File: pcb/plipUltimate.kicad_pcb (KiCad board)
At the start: 2 copper layers, 50 x 50 mm, 55 parts, among them CON1 IEEEE-1284A, CON2 AVR-ISP-6, CON3 RJ45_C, CON4 SD_SPI, CON5 USB_microB, U1 ENC28J60, U2 ATMEGA328P, U3 LM2596_5.0, U4 74LS07, U5 IRF7309, U6 AMS1117_3V3, U7 IRF7309, X1 25MHz

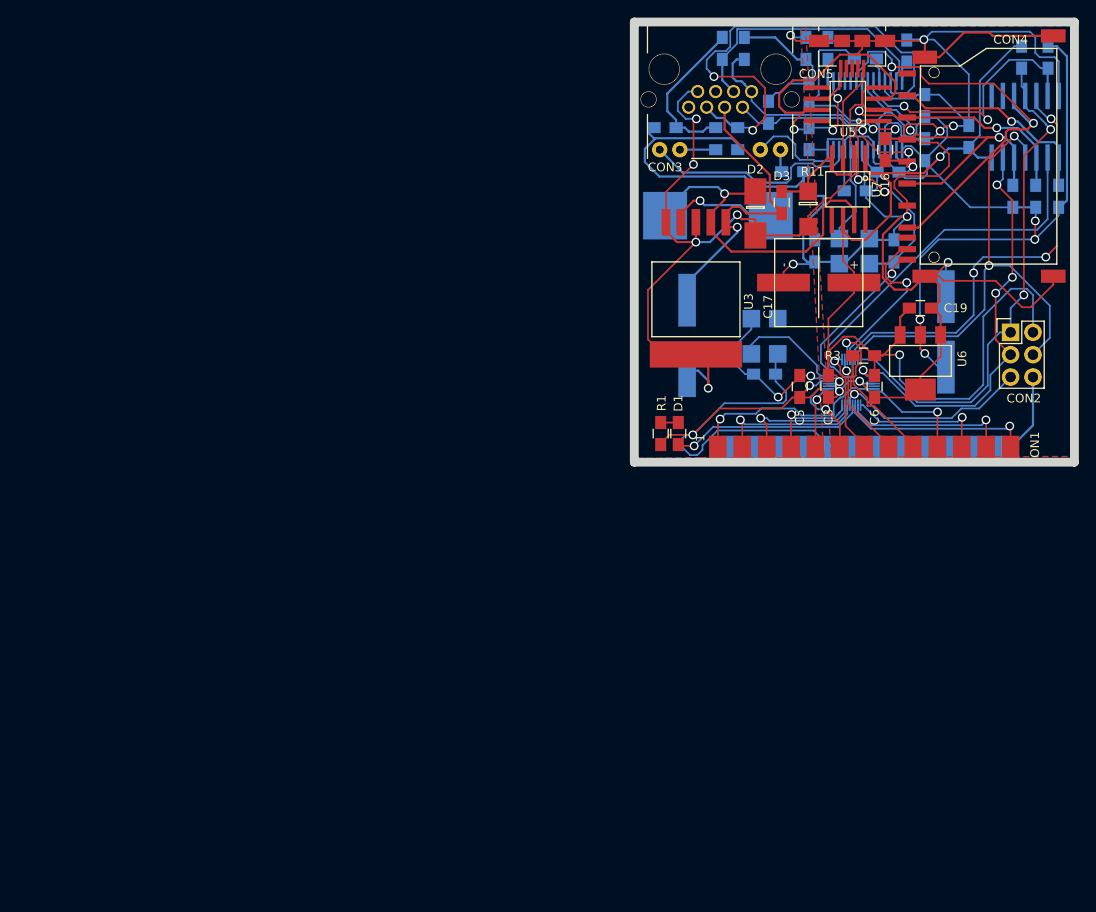
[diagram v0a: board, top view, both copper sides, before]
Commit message: Revised schematic, reroute in progress
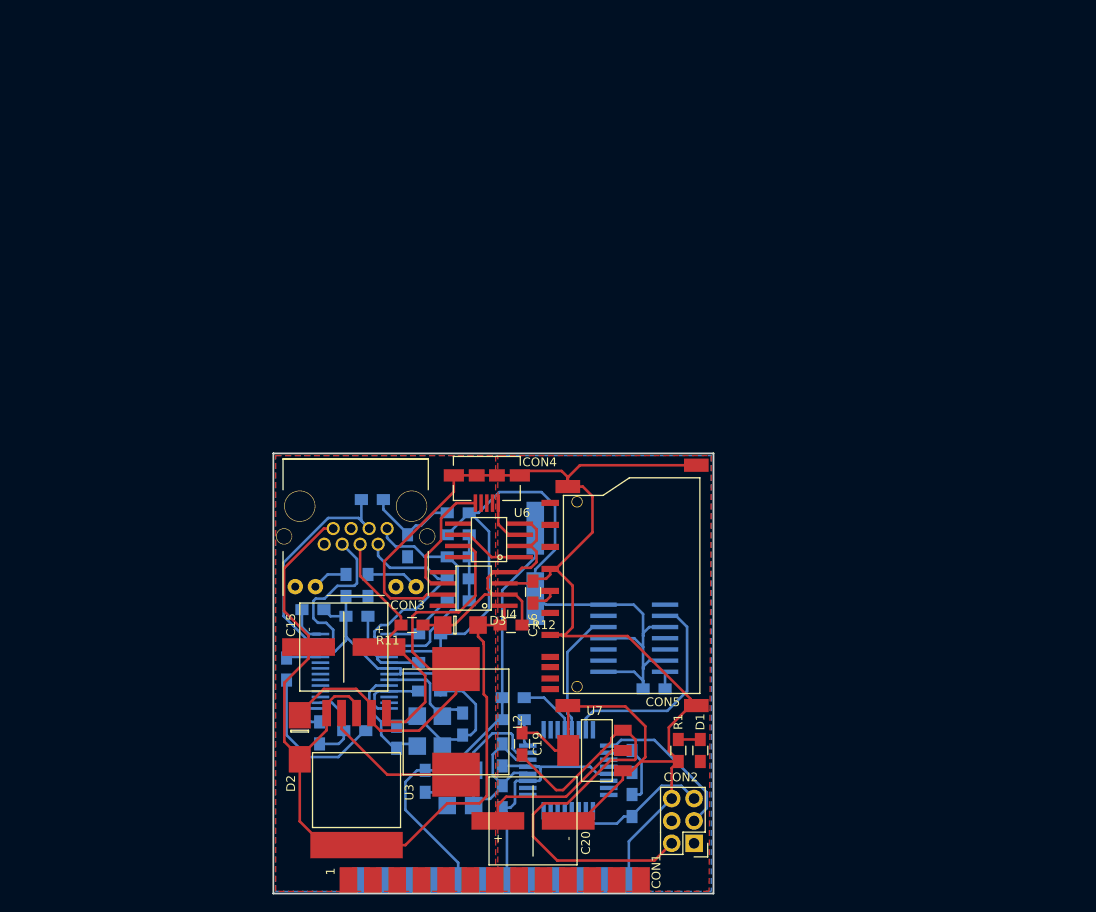
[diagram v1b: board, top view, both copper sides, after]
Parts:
- removed R15, R16: 1k, plipUltimate:0805
- C15, C20, L2: moved to F.Cu
- C17: value 220uF 35V loESR -> 10nF; footprint plipUltimate:electrolyte_SMD -> plipUltimate:0805; moved to B.Cu
- C18: value 10nF -> 220uF 35V loESR; footprint plipUltimate:0805 -> plipUltimate:electrolyte_SMD
- C3, C5, C6, R3: moved to B.Cu
- CON4: value SD_SPI -> USB_microB; footprint plipUltimate:SD-SHORT -> plipUltimate:USB-MicroB
- CON5: value USB_microB -> SD_SPI; footprint plipUltimate:USB-MicroB -> plipUltimate:SD-SHORT
- R1: value 330R -> 820R
- R12: value 1k -> 10k; moved to F.Cu
- R13, R14: value 1k -> 4k7
- U2: footprint plipUltimate:TQFP_32 -> plipUltimate:TQFP-32
- U4: value 74LS07 -> IRF7309; footprint plipUltimate:SO-14 -> plipUltimate:SO-8; moved to F.Cu
- U5: value IRF7309 -> 74LVC125; footprint plipUltimate:SO-8 -> plipUltimate:SO-14; moved to B.Cu
- U6: value AMS1117_3V3 -> IRF7309; footprint plipUltimate:SOT-223 -> plipUltimate:SO-8
- U7: value IRF7309 -> AMS1117_3V3; footprint plipUltimate:SO-8 -> plipUltimate:SOT-223
- moved C8 96.9 mm to (84.2, 120.8), turned to 90 degrees
- moved R13 96.7 mm to (106.2, 119.2), turned to 0 degrees
- moved R4 95.5 mm to (80.5, 113.5), turned to 90 degrees
- moved R2 92.6 mm to (83.5, 106.8), turned to 0 degrees
- moved C2 86.7 mm to (88.5, 107.5), turned to 0 degrees
- moved R12 86.7 mm to (106.0, 108.5), turned to 0 degrees
- moved U1 85.7 mm to (88.2, 113.8), turned to 90 degrees
- moved C1 84.8 mm to (88.2, 120.5), turned to 0 degrees
- moved R14 84.1 mm to (106.2, 116.8), turned to 0 degrees
- moved U4 80.1 mm to (104.2, 106.3), turned to 90 degrees
- moved D2 78.9 mm to (82.0, 121.2)
- moved C4 78.7 mm to (96.8, 109.5), turned to 180 degrees
- moved CON5 78.2 mm to (111.5, 115.8), turned to 90 degrees
- moved C7 76.3 mm to (96.8, 112.8), turned to 180 degrees
- moved C9 74.6 mm to (96.8, 116.0)
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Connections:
- C17 pad 1: +5V -> +3V3
- C18 pad 1: GND -> +5V
- C18 pad 2: +5V -> GND
- CON4 pad 1: 3.3V_SD_CS -> Net-(CON4-Pad1)
- CON4 pad 2: 3.3V_AVR_MOSI -> Net-(CON4-Pad2)
- CON4 pad 3: GND -> Net-(CON4-Pad3)
- CON4 pad 4: +3V3 -> Net-(CON4-Pad4)
- CON4 pad 5: 3.3V_AVR_SCK -> Net-(CON4-Pad5)
- CON5 pad 1: Net-(CON5-Pad1) -> 3.3V_SD_CS
- CON5 pad 2: Net-(CON5-Pad2) -> 3.3V_AVR_MOSI
- CON5 pad 3: Net-(CON5-Pad3) -> GND
- CON5 pad 4: Net-(CON5-Pad4) -> +3V3
- CON5 pad 5: Net-(CON5-Pad5) -> 3.3V_AVR_SCK
- R12 pad 1: +5V -> POE_0V
- R12 pad 2: AVR_MISO -> Net-(D3-Pad1)
- R13 pad 1: +3V3 -> +5V
- R13 pad 2: 3.3V_ETH_CS -> SD_DETECT
- R14 pad 1: +3V3 -> +5V
- R14 pad 2: 3.3V_SD_CS -> SD_LOCK
- U1 pad 6: 3.3V_AVR_MISO -> AVR_MISO
- U1 pad 7: 3.3V_AVR_MOSI -> AVR_MOSI
- U1 pad 8: 3.3V_AVR_SCK -> AVR_SCK
- U1 pad 9: 3.3V_ETH_CS -> ETH_CS
- U4 pad 1: Net-(U4-Pad1) -> POE_0V
- U4 pad 2: Net-(U4-Pad2) -> Net-(D3-Pad1)
- U4 pad 3: 3.3V_AVR_MISO -> GND
- U4 pad 4: AVR_MISO -> Net-(D3-Pad1)
- U4 pad 5: ETH_CS -> (no net)
- U4 pad 6: 3.3V_ETH_CS -> Net-(CON4-Pad5)
- U4 pad 8: 3.3V_SD_CS -> (no net)
- U5 pad 1: POE_0V -> GND
- U5 pad 2: Net-(D3-Pad1) -> Net-(U5-Pad2)
- U5 pad 3: GND -> Net-(U5-Pad3)
- U5 pad 4: Net-(D3-Pad1) -> GND
- U5 pad 5: (no net) -> SD_CS
- U5 pad 6: Net-(CON5-Pad5) -> 3.3V_SD_CS
- U5 pad 8: (no net) -> 3.3V_AVR_MOSI
- U6 pad 1: GND -> +5V
- U6 pad 2: +3V3 -> Net-(D3-Pad1)
- U6 pad 3: +5V -> Net-(CON4-Pad1)
- U7 pad 1: +5V -> GND
- U7 pad 2: Net-(D3-Pad1) -> +3V3
- U7 pad 3: Net-(CON5-Pad1) -> +5V
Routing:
- net +3V3: track 150.2 -> 68.0 mm, vias 5 -> 0
- net AVR_MISO: track 58.9 -> 0.00 mm, vias 2 -> 0
- net 3.3V_AVR_MISO: track 51.6 -> 0.00 mm, vias 2 -> 0
- net ETH_CS: track 51.5 -> 0.00 mm, vias 3 -> 0
- net 3.3V_AVR_SCK: track 37.9 -> 0.00 mm, vias 2 -> 0
- net Net-(CON3-Pad6): track 56.3 -> 18.8 mm, vias 2 -> 0
- net AVR_MOSI: track 56.5 -> 24.4 mm, vias 2 -> 0
- net 3.3V_ETH_CS: track 31.7 -> 0.00 mm, vias 2 -> 0
- net SD_CS: track 45.2 -> 14.4 mm
- net 3.3V_AVR_MOSI: track 30.6 -> 0.00 mm, vias 2 -> 0
- net AVR_SCK: track 45.4 -> 18.7 mm, vias 3 -> 0
- net /~STROBE: track 26.6 -> 0.00 mm, vias 1 -> 0
- net GND: track 430.3 -> 404.5 mm, vias 14 -> 0
- net Net-(CON3-Pad12): track 25.2 -> 0.00 mm
- net 3.3V_SD_CS: track 24.0 -> 0.00 mm, vias 1 -> 0
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- added copper zone on B.Cu, net GND
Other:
- net class Default: clearance 0.1 -> 0.3; trace_width 0.2 -> 0.3; via_dia 1 -> 1.5; via_drill 0.7 -> 0.3
- rule pad_to_mask_clearance: 0.2 -> 0
- rule trace_clearance: 0.1 -> 0.3
- rule via_min_size: 1 -> 0.4
- board text added: "BS: Children of the grave Rev. 2"
- board text added: "github.com/tehKaiN/plipUltimate"

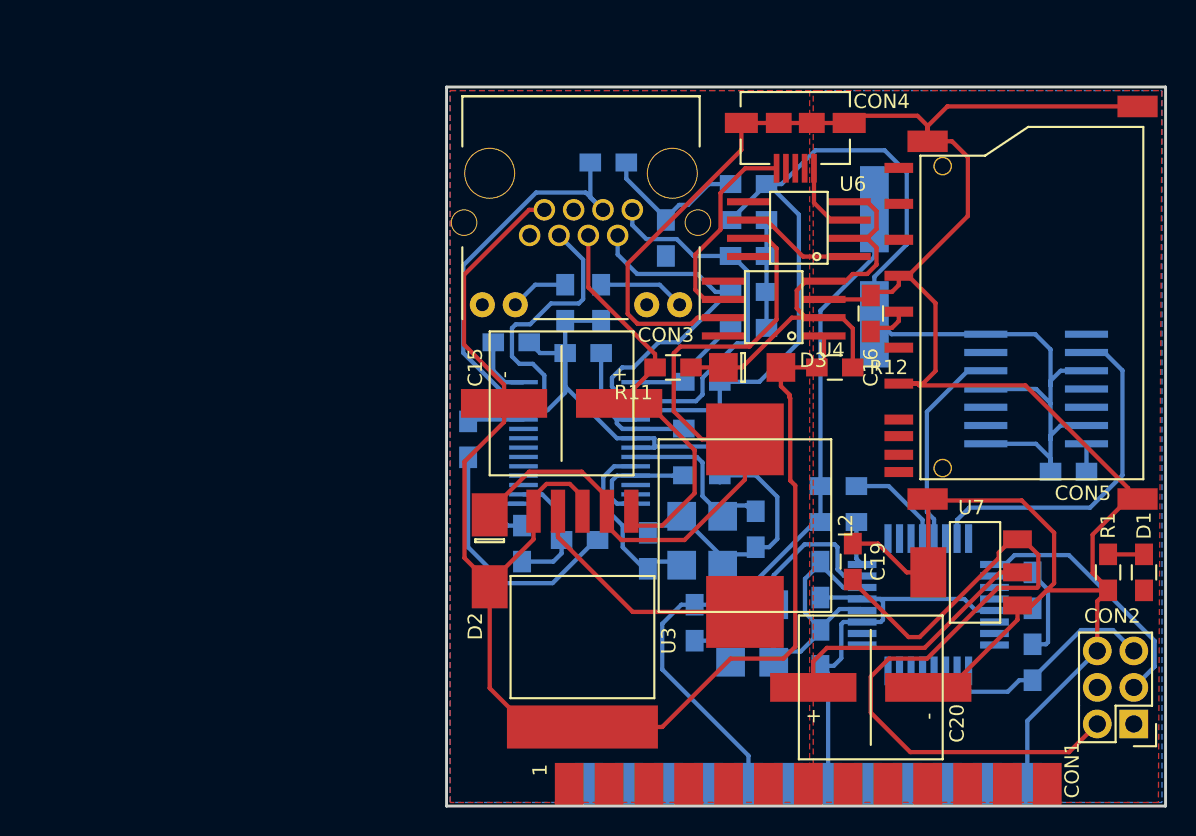
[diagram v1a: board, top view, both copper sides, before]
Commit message: Complete rev 2 sch and PCB
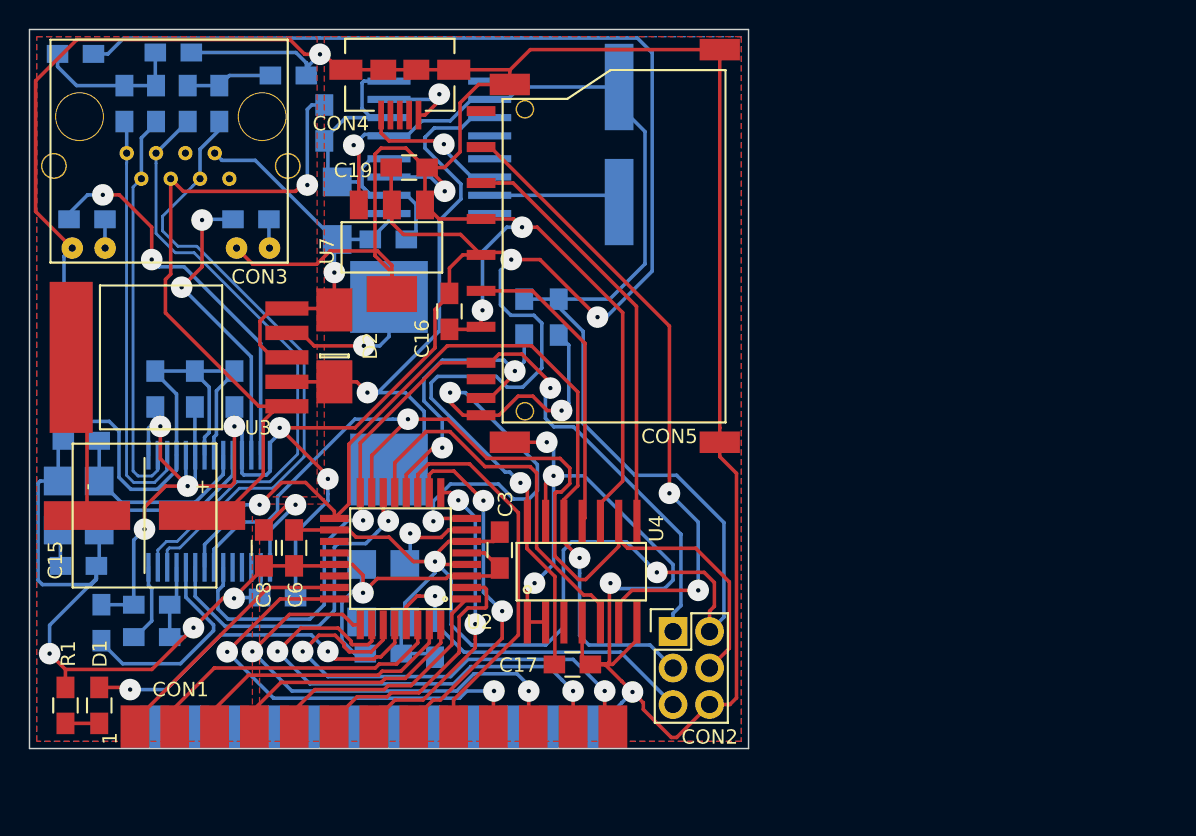
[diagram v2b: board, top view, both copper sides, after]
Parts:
- removed C20: 47uF 6,3V, plipUltimate:electrolyte_SMD
- removed C5: 100nF, plipUltimate:0805
- C17, C3, C6, C8, U2: moved to F.Cu
- C19: value 100nF -> 10uF 6,3V
- D3, L2, R11, R12, U6: moved to B.Cu
- U4: value IRF7309 -> 74LVC125; footprint plipUltimate:SO-8 -> plipUltimate:SO-14
- U5: value 74LVC125 -> IRF7309; footprint plipUltimate:SO-14 -> plipUltimate:SO-8
- moved D1 73.2 mm to (54.9, 132.0), turned to 90 degrees
- moved R1 73.1 mm to (52.5, 132.0), turned to 90 degrees
- moved C6 51.4 mm to (68.4, 121.0)
- moved L1 50.5 mm to (53.2, 86.7), turned to 180 degrees
- moved U7 48.8 mm to (75.2, 98.4), turned to 180 degrees
- moved C11 47.3 mm to (53.6, 113.6), turned to 0 degrees
- moved R5 44.7 mm to (56.6, 90.2), turned to 270 degrees
- moved U5 44.5 mm to (76.0, 97.8)
- moved X1 43.4 mm to (53.4, 118.1)
- moved R6 43.2 mm to (58.8, 90.2), turned to 270 degrees
- moved U3 41.8 mm to (54.4, 107.8), turned to 90 degrees
- moved C12 41.7 mm to (60.0, 86.6), turned to 180 degrees
- moved R3 41.6 mm to (78.2, 127.4), turned to 90 degrees
- moved C19 41.3 mm to (76.4, 94.6), turned to 0 degrees
- moved C10 39.6 mm to (53.4, 122.3), turned to 180 degrees
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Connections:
- net Net-(C10-Pad2) renamed /OSC2
- net Net-(C11-Pad2) renamed /OSC1
- net Net-(CON3-Pad1) renamed /TX+
- net Net-(CON3-Pad2) renamed /TX-
- net Net-(CON3-Pad3) renamed /RX+
- net Net-(CON3-Pad6) renamed /RX-
- net Net-(G1-Pad3) renamed /AVR_CLK
- C19 pad 1: +5V -> +3V3
- CON3 pad 11: Net-(CON3-Pad11) -> GND
- CON3 pad 9: Net-(CON3-Pad9) -> GND
- R10 pad 1: Net-(CON3-Pad11) -> Net-(CON3-Pad12)
- R10 pad 2: GND -> /LEDB
- R9 pad 1: Net-(CON3-Pad9) -> Net-(CON3-Pad10)
- R9 pad 2: GND -> /LEDA
- U1 pad 26: Net-(CON3-Pad12) -> /LEDB
- U1 pad 27: Net-(CON3-Pad10) -> /LEDA
- U4 pad 1: POE_0V -> GND
- U4 pad 2: Net-(D3-Pad1) -> GND
- U4 pad 3: GND -> Net-(U4-Pad3)
- U4 pad 4: Net-(D3-Pad1) -> GND
- U4 pad 5: (no net) -> SD_CS
- U4 pad 6: Net-(CON4-Pad5) -> 3.3V_SD_CS
- U4 pad 8: (no net) -> 3.3V_AVR_MOSI
- U5 pad 1: GND -> POE_0V
- U5 pad 2: Net-(U5-Pad2) -> Net-(D3-Pad1)
- U5 pad 3: Net-(U5-Pad3) -> GND
- U5 pad 4: GND -> Net-(D3-Pad1)
- U5 pad 5: SD_CS -> (no net)
- U5 pad 6: 3.3V_SD_CS -> Net-(CON4-Pad5)
- U5 pad 8: 3.3V_AVR_MOSI -> (no net)
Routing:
- net +3V3: track 68.0 -> 209.0 mm, vias 0 -> 9
- net AVR_MISO: track 0.00 -> 63.2 mm, vias 0 -> 2
- net POE_0V: track 101.0 -> 41.5 mm, vias 0 -> 1
- net GND: track 404.5 -> 453.4 mm, vias 0 -> 13
- net AVR_SCK: track 18.7 -> 65.9 mm, vias 0 -> 2
- net AVR_MOSI: track 24.4 -> 69.2 mm, vias 0 -> 1
- net 3.3V_SD_CS: track 0.00 -> 44.7 mm, vias 0 -> 2
- net /POUT: track 0.00 -> 34.7 mm, vias 0 -> 2
- net SD_DETECT: track 3.12 -> 37.7 mm, vias 0 -> 3
- net /SEL: track 0.00 -> 34.4 mm, vias 0 -> 2
- net /BUSY: track 0.00 -> 33.6 mm, vias 0 -> 2
- net /~ACK: track 0.00 -> 31.6 mm, vias 0 -> 2
- net 3.3V_AVR_MOSI: track 0.00 -> 29.3 mm
- net /LEDA: track 0.00 -> 27.6 mm, vias 0 -> 2
- net /D7: track 0.00 -> 27.2 mm
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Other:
- net class Default: clearance 0.3 -> 0.25; trace_width 0.3 -> 0.25
- rule trace_clearance: 0.3 -> 0.25
- rule via_min_size: 0.4 -> 1.5
- board text added: "Children of the Grave plipUltimate Rev. 2"
- board text removed: "BS: Children of the grave Rev. 2"
- board text removed: "github.com/tehKaiN/plipUltimate"
